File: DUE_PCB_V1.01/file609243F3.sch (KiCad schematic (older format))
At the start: 24 parts, among them J29 Motor_Right1, J30 Motor_Right2, J31 Motor_Left1, J32 Motor_Left2, J33 Cutter_Motor, J34 ODORight1, J35 ODORight2, J36 ODOLeft1, J37 ODOLeft2, J38 ODOCutter

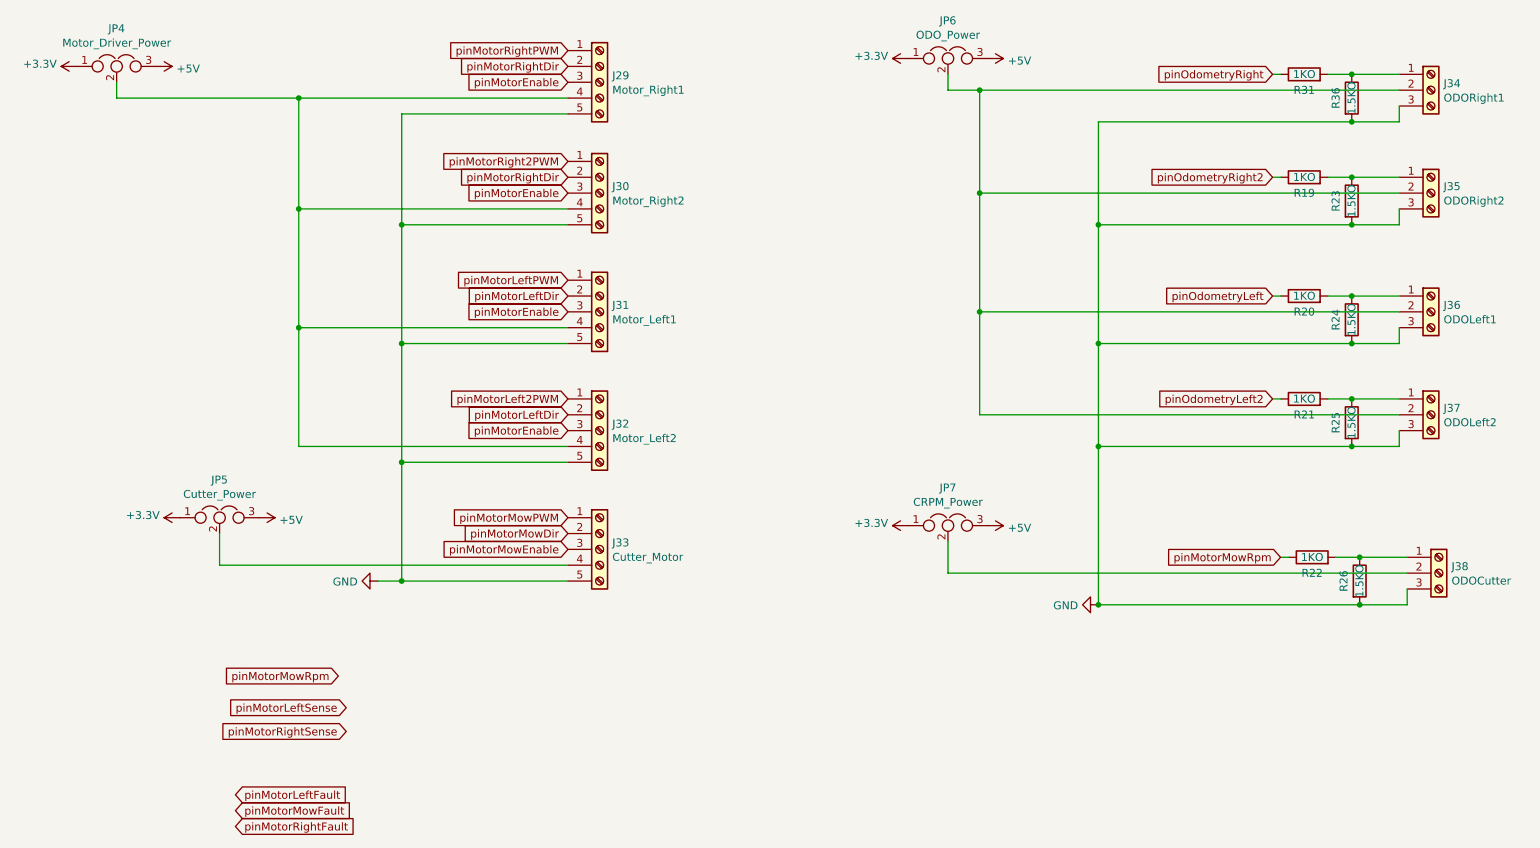
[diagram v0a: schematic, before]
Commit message: first test
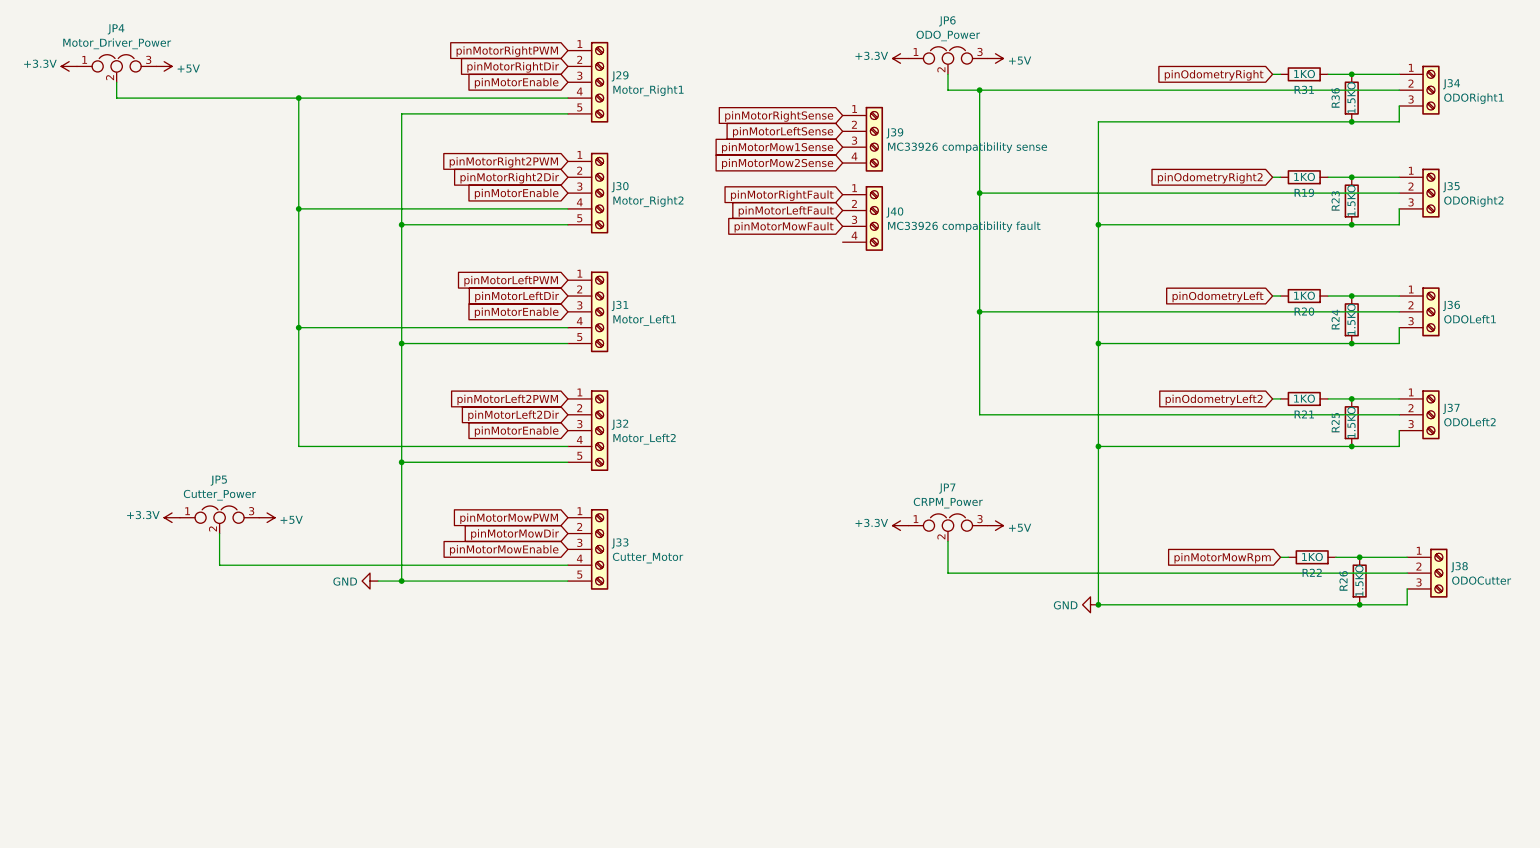
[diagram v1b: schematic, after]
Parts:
- added J39: MC33926 compatibility sense, Connector_JST:JST_XH_B4B-XH-A_1x04_P2.50mm_Vertical, symbol Connector:Screw_Terminal_01x04
- added J40: MC33926 compatibility fault, Connector_JST:JST_XH_B4B-XH-A_1x04_P2.50mm_Vertical, symbol Connector:Screw_Terminal_01x04
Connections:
- net pinMotorLeftDir: no longer J32.2 (Pin_2)
- net pinMotorLeftFault: now also J40.2 (Pin_2)
- net pinMotorLeftSense: now also J39.2 (Pin_2)
- net pinMotorMowFault: now also J40.3 (Pin_3)
- net pinMotorRightDir: no longer J30.2 (Pin_2)
- net pinMotorRightFault: now also J40.1 (Pin_1)
- net pinMotorRightSense: now also J39.1 (Pin_1)
- new net pinMotorLeft2Dir: J32.2 (Pin_2)
- new net pinMotorMow1Sense: J39.3 (Pin_3)
- new net pinMotorMow2Sense: J39.4 (Pin_4)
- new net pinMotorRight2Dir: J30.2 (Pin_2)
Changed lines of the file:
@@
 Text GLabel 4150 4050 0    50   Input ~ 0
 pinMotorMowEnable
-Text GLabel 4150 1700 0    50   Input ~ 0
-pinMotorRightDir
-Text GLabel 4150 3200 0    50   Input ~ 0
-pinMotorLeftDir
 $Comp
 L power:GND #PWR?
@@
 Wire Wire Line
 	3100 4250 4150 4250
-Text GLabel 2750 5050 0    50   Input ~ 0
-pinMotorLeftSense
-Text GLabel 2750 5200 0    50   Input ~ 0
-pinMotorRightSense
-Text GLabel 2050 5800 2    50   Input ~ 0
+Text GLabel 5885 1810 0    50   Input ~ 0
 pinMotorRightFault
-Text GLabel 2050 5600 2    50   Input ~ 0
+Text GLabel 5885 1910 0    50   Input ~ 0
 pinMotorLeftFault
-Text GLabel 2050 5700 2    50   Input ~ 0
-pinMotorMowFault
-Text GLabel 2700 4850 0    50   Input ~ 0
-pinMotorMowRpm
 Text GLabel 4150 1800 0    50   Input ~ 0
 pinMotorEnable
@@
 Text GLabel 4150 3300 0    50   Input ~ 0
 pinMotorEnable
+Text GLabel 4150 3200 0    50   Input ~ 0
+pinMotorLeft2Dir
+Text GLabel 4150 1700 0    50   Input ~ 0
+pinMotorRight2Dir
+Text GLabel 5885 1310 0    50   Input ~ 0
+pinMotorRightSense
+Text GLabel 5885 1410 0    50   Input ~ 0
+pinMotorLeftSense
+Text GLabel 5885 2010 0    50   Input ~ 0
+pinMotorMowFault
+Text GLabel 5885 1510 0    50   Input ~ 0
+pinMotorMow1Sense
+Text GLabel 5885 1610 0    50   Input ~ 0
+pinMotorMow2Sense
+$Comp
+L Connector:Screw_Terminal_01x04 J39
+U 1 1 60A7B735
+P 6085 1410
+F 0 "J39" H 6165 1402 50  0000 L CNN
+F 1 "MC33926 compatibility sense" H 6165 1311 50  0000 L CNN
+F 2 "Connector_JST:JST_XH_B4B-XH-A_1x04_P2.50mm_Vertical" H 6085 1410 50  0001 C CNN
+F 3 "~" H 6085 1410 50  0001 C CNN
+	1    6085 1410
+	1    0    0    -1
+$EndComp
+$Comp
+L Connector:Screw_Terminal_01x04 J40
+U 1 1 60A825D0
+P 6085 1910
+F 0 "J40" H 6165 1902 50  0000 L CNN
+F 1 "MC33926 compatibility fault" H 6165 1811 50  0000 L CNN
+F 2 "Connector_JST:JST_XH_B4B-XH-A_1x04_P2.50mm_Vertical" H 6085 1910 50  0001 C CNN
+F 3 "~" H 6085 1910 50  0001 C CNN
+	1    6085 1910
+	1    0    0    -1
+$EndComp
 $EndSCHEMATC
